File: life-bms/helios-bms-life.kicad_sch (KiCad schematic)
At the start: 55 parts, among them J1 Outboard, J2 Debug, J3 Output, J4 Battery, Q1 SSM3J332R, Q2 Q_Dual_NMOS_PMOS_S1G1D2S2G2D1, Q3 PMOS, U1 TPSM861253, U2 BQ25306, U3 STM32L011F4Ux, U4 THVD1400D, U5 SIP32434

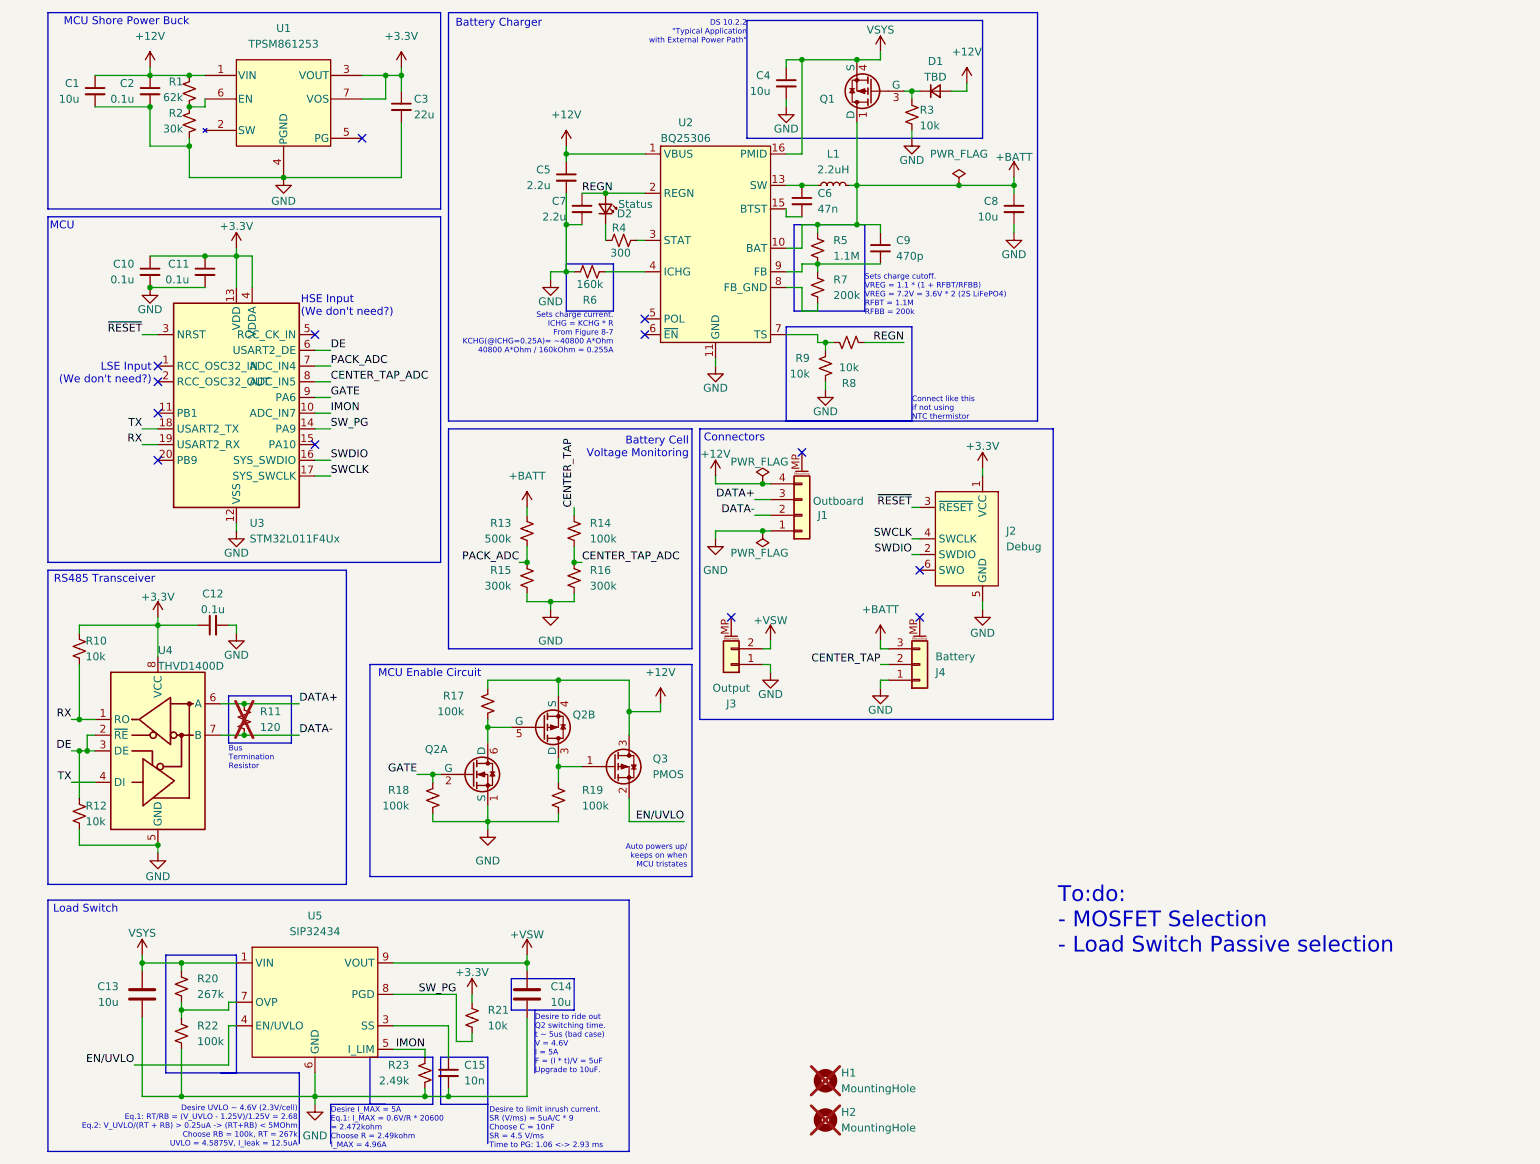
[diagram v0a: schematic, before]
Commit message: oops
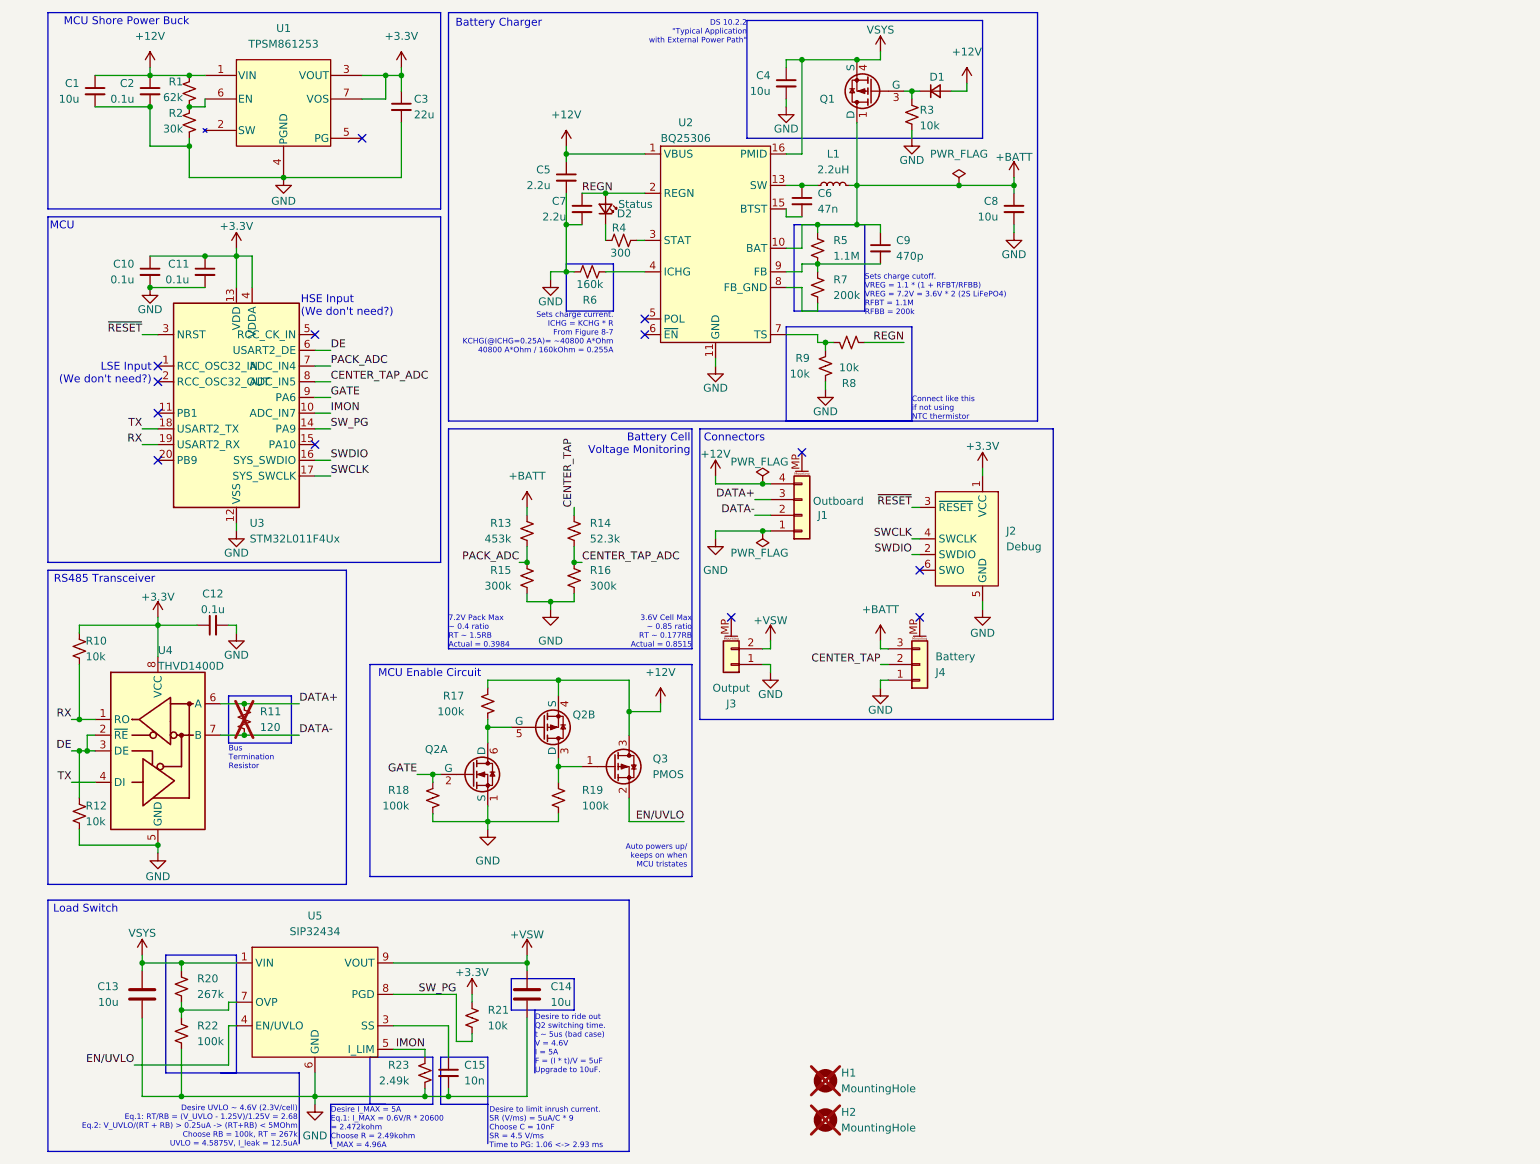
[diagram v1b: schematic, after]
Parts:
- D1: value TBD -> GSDH3005
- Q1: value SSM3J332R -> SSM6J507NU
- R13: value 500k -> 453k
- R14: value 100k -> 52.3k
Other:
- note added: "3.6V Cell Max ~ 0.85 ratio RT ~ 0.177RB Actual = 0.8515"
- note added: "7.2V Pack Max ~ 0.4 ratio RT ~ 1.5RB Actual = 0.3984"
- note removed: "To:do: - MOSFET Selection - Load Switch Passive selection"
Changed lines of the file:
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@@
 		)
 	)
-	(text "To:do:\n- MOSFET Selection\n- Load Switch Passive selection"
-		(exclude_from_sim no)
-		(at 177.292 160.782 0)
-		(effects
-			(font
-				(size 2.54 2.54)
-			)
-			(justify left)
-		)
-	)
 	(text "DS 10.2.2\n\"Typical Application\nwith External Power Path\""
 		(exclude_from_sim no)
@@
 	(text "Battery Cell\nVoltage Monitoring"
 		(exclude_from_sim no)
-		(at 117.602 84.328 0)
+		(at 117.856 83.82 0)
 		(effects
 			(font
@@
 		)
 	)
+	(text "7.2V Pack Max\n~ 0.4 ratio\nRT ~ 1.5RB\nActual = 0.3984"
+		(exclude_from_sim no)
+		(at 78.74 116.84 0)
+		(effects
+			(font
+				(size 0.889 0.889)
+				(color 0 0 0 1)
+			)
+			(justify left bottom)
+		)
+	)
 	(text "Battery Charger"
 		(exclude_from_sim no)
@@
 		)
 	)
+	(text "3.6V Cell Max\n~ 0.85 ratio\nRT ~ 0.177RB\nActual = 0.8515"
+		(exclude_from_sim no)
+		(at 118.11 116.84 0)
+		(effects
+			(font
+				(size 0.889 0.889)
+				(color 0 0 0 1)
+			)
+			(justify right bottom)
+		)
+	)
 	(text "Connectors"
 		(exclude_from_sim no)
@@
 			)
 		)
-		(property "Value" "500k"
+		(property "Value" "453k"
 			(at 88.9 99.0599 0)
 			(show_name no)
@@
 			)
 		)
-		(property "Value" "SSM3J332R"
+		(property "Value" "SSM6J507NU"
 			(at 141.224 25.4 90)
 			(hide yes)
@@
 		(dnp no)
 		(property "Reference" "D1"
-			(at 157.48 21.844 0)
+			(at 157.734 24.384 0)
 			(show_name no)
 			(do_not_autoplace no)
@@
 			)
 		)
-		(property "Value" "TBD"
+		(property "Value" "GSDH3005"
 			(at 157.48 24.384 0)
+			(hide yes)
 			(show_name no)
 			(do_not_autoplace no)
@@
 			)
 		)
-		(property "Value" "100k"
+		(property "Value" "52.3k"
 			(at 101.6 99.0599 0)
 			(show_name no)

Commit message: update BoM
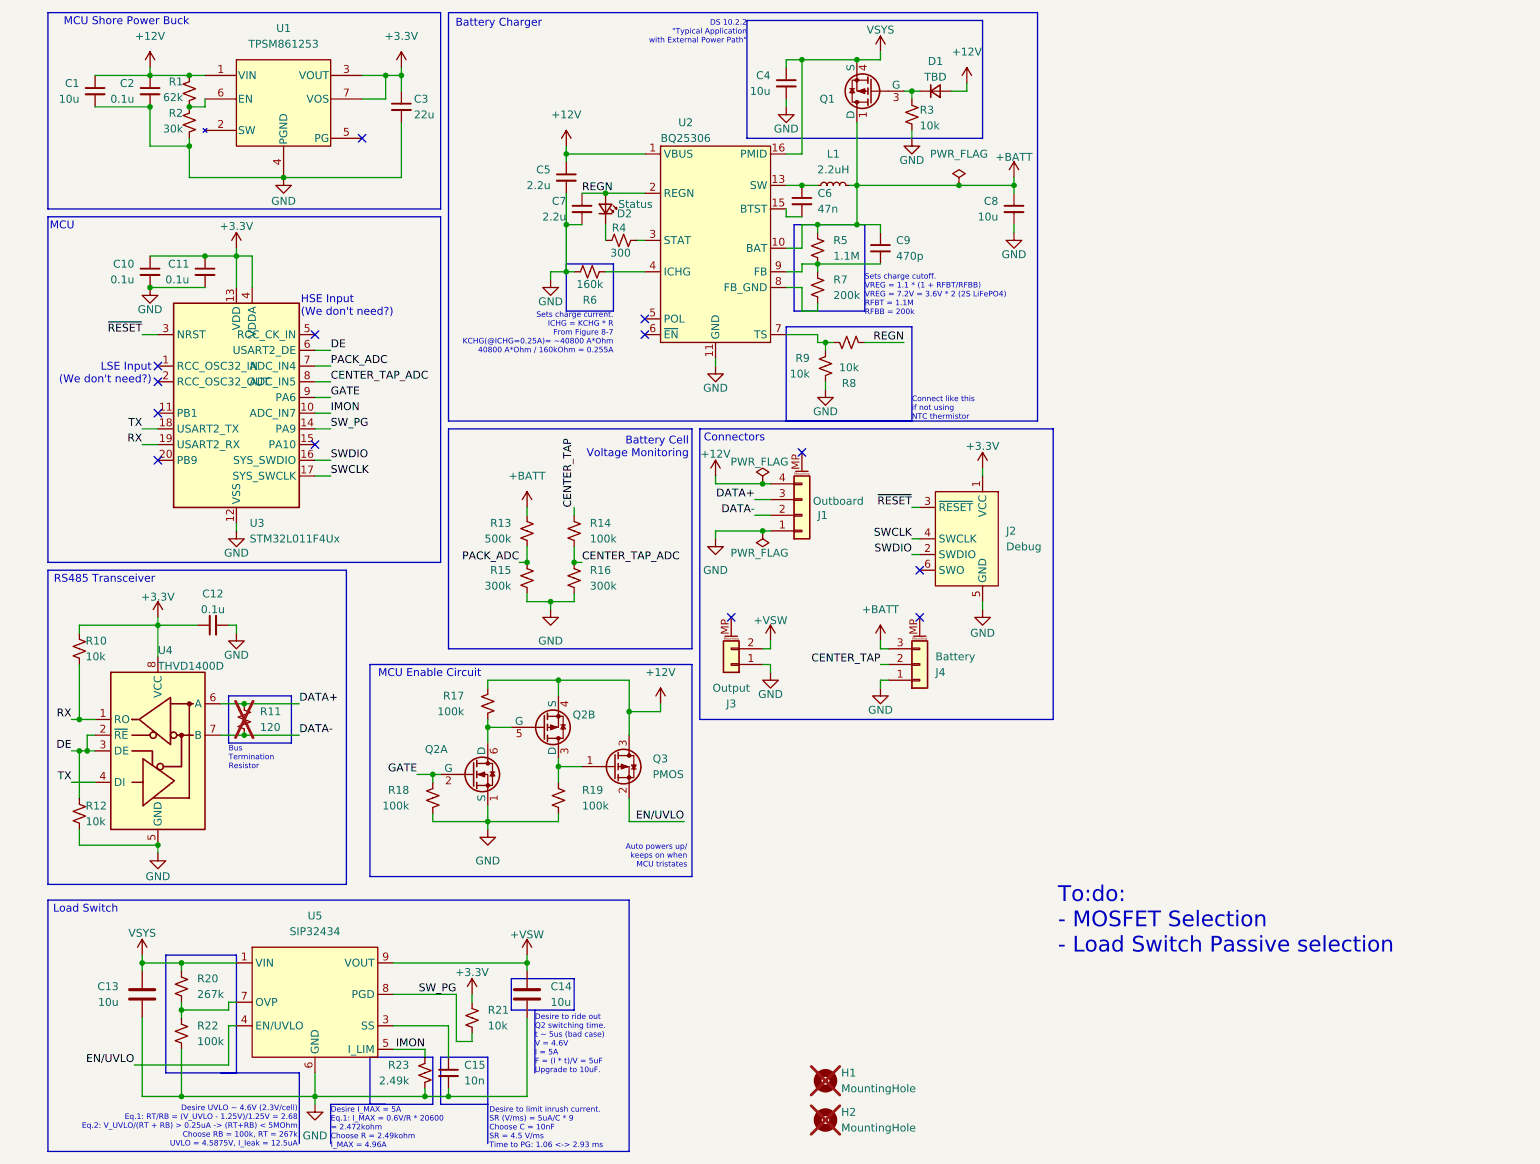
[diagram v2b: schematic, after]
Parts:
- D1: value GSDH3005 -> TBD
- Q1: value SSM6J507NU -> SSM3J332R
- R13: value 453k -> 500k
- R14: value 52.3k -> 100k
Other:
- note added: "To:do: - MOSFET Selection - Load Switch Passive selection"
- note removed: "3.6V Cell Max ~ 0.85 ratio RT ~ 0.177RB Actual = 0.8515"
- note removed: "7.2V Pack Max ~ 0.4 ratio RT ~ 1.5RB Actual = 0.3984"
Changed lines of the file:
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@@
 		)
 	)
+	(text "To:do:\n- MOSFET Selection\n- Load Switch Passive selection"
+		(exclude_from_sim no)
+		(at 177.292 160.782 0)
+		(effects
+			(font
+				(size 2.54 2.54)
+			)
+			(justify left)
+		)
+	)
 	(text "DS 10.2.2\n\"Typical Application\nwith External Power Path\""
 		(exclude_from_sim no)
@@
 	(text "Battery Cell\nVoltage Monitoring"
 		(exclude_from_sim no)
-		(at 117.856 83.82 0)
+		(at 117.602 84.328 0)
 		(effects
 			(font
@@
 		)
 	)
-	(text "7.2V Pack Max\n~ 0.4 ratio\nRT ~ 1.5RB\nActual = 0.3984"
-		(exclude_from_sim no)
-		(at 78.74 116.84 0)
-		(effects
-			(font
-				(size 0.889 0.889)
-				(color 0 0 0 1)
-			)
-			(justify left bottom)
-		)
-	)
 	(text "Battery Charger"
 		(exclude_from_sim no)
@@
 		)
 	)
-	(text "3.6V Cell Max\n~ 0.85 ratio\nRT ~ 0.177RB\nActual = 0.8515"
-		(exclude_from_sim no)
-		(at 118.11 116.84 0)
-		(effects
-			(font
-				(size 0.889 0.889)
-				(color 0 0 0 1)
-			)
-			(justify right bottom)
-		)
-	)
 	(text "Connectors"
 		(exclude_from_sim no)
@@
 			)
 		)
-		(property "Value" "453k"
+		(property "Value" "500k"
 			(at 88.9 99.0599 0)
 			(show_name no)
@@
 			)
 		)
-		(property "Value" "SSM6J507NU"
+		(property "Value" "SSM3J332R"
 			(at 141.224 25.4 90)
 			(hide yes)
@@
 		(dnp no)
 		(property "Reference" "D1"
-			(at 157.734 24.384 0)
+			(at 157.48 21.844 0)
 			(show_name no)
 			(do_not_autoplace no)
@@
 			)
 		)
-		(property "Value" "GSDH3005"
+		(property "Value" "TBD"
 			(at 157.48 24.384 0)
-			(hide yes)
 			(show_name no)
 			(do_not_autoplace no)
@@
 			)
 		)
-		(property "Value" "52.3k"
+		(property "Value" "100k"
 			(at 101.6 99.0599 0)
 			(show_name no)
